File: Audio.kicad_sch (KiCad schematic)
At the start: 2 parts, among them J3 AudioJack3_Ground_SwitchTR, U3 WM8960CGEFL/RV

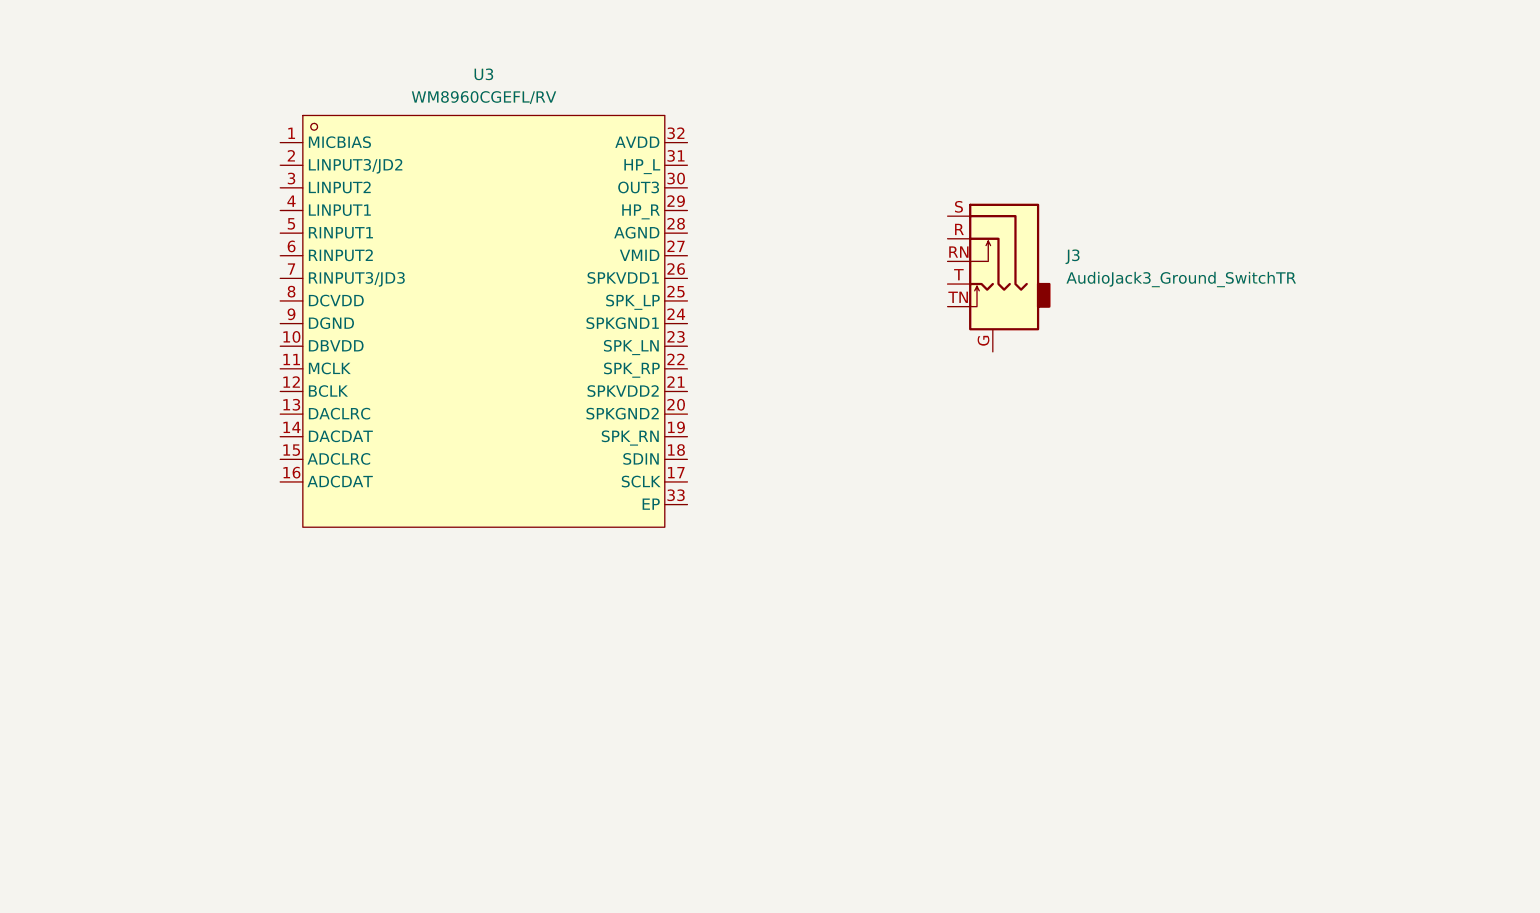
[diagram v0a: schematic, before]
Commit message: audio and display changes
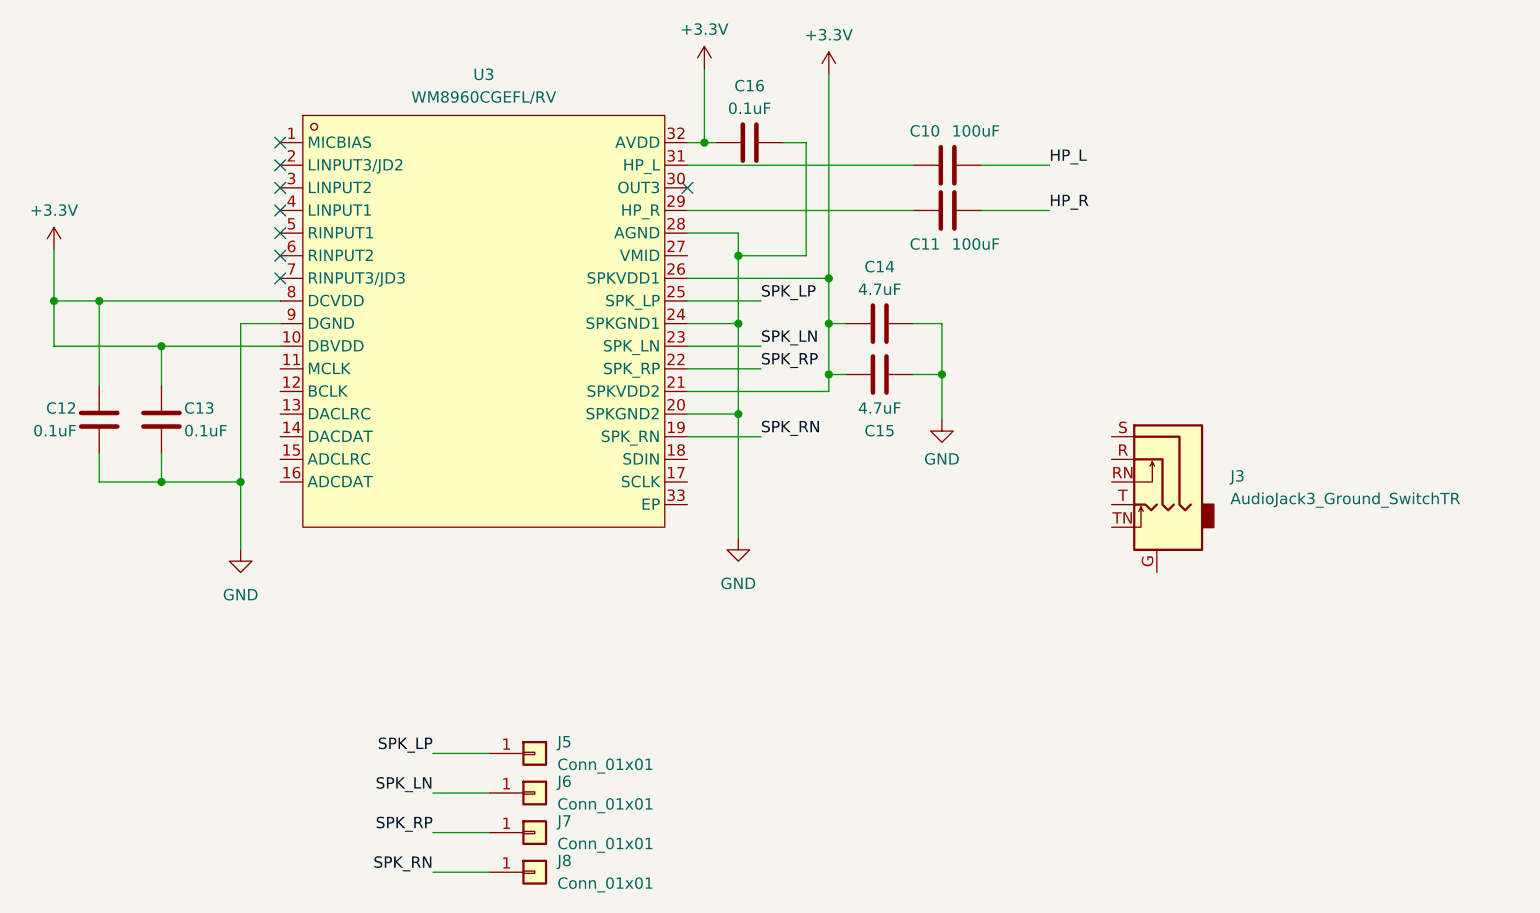
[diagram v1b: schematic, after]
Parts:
- added C10, C11: 100uF, symbol Device:C
- added C12, C13, C16: 0.1uF, symbol Device:C
- added C14, C15: 4.7uF, symbol Device:C
- added J5, J6, J7, J8: Conn_01x01, symbol Connector_Generic:Conn_01x01
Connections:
- net +3.3V: now reaches U3.10 (DBVDD)
- net +3.3V: now also U3.21 (SPKVDD2), U3.26 (SPKVDD1), U3.32 (AVDD), U3.8 (DCVDD), C12.1, C13.1, C14.1, C15.1, C16.1
- net SPK_RN: now reaches U3.19 (SPK_RN)
- net SPK_RN: now also J8.1 (Pin_1)
- net GND: now reaches U3.20 (SPKGND2)
- net GND: now also U3.24 (SPKGND1), U3.28 (AGND), U3.9 (DGND), C12.2, C13.2, C14.2, C15.2, C16.2
- net SPK_RP: now reaches U3.22 (SPK_RP)
- net SPK_RP: now also J7.1 (Pin_1)
- net SPK_LN: now reaches U3.23 (SPK_LN)
- net SPK_LN: now also J6.1 (Pin_1)
- net SPK_LP: now reaches U3.25 (SPK_LP)
- net SPK_LP: now also J5.1 (Pin_1)
- net at U3.29 (HP_R): now also C11.2
- net at U3.31 (HP_L): now also C10.1
- new net HP_L: C10.2
- new net HP_R: C11.1
- no-connect marks 0 -> 8
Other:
- moved on the sheet: J3

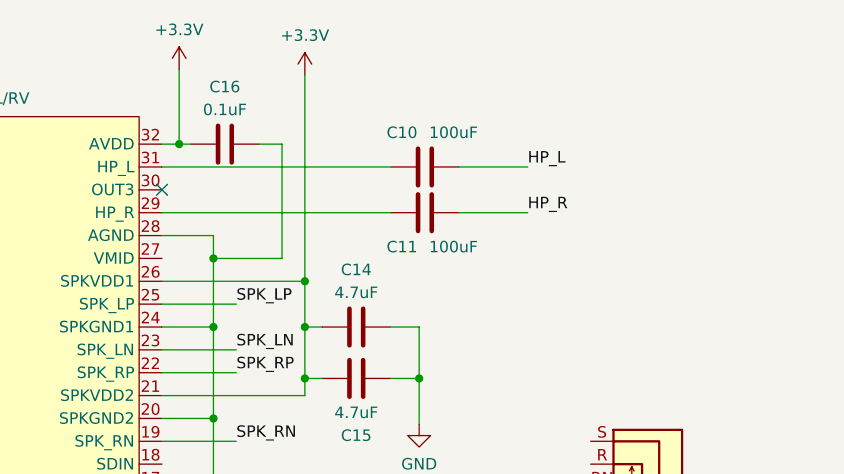
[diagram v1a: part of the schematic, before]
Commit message: more display things
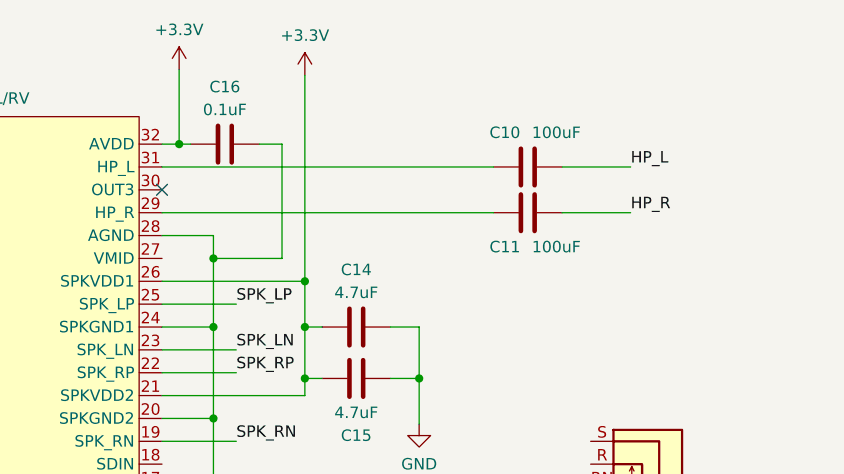
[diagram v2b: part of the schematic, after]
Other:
- moved on the sheet: C10, C11
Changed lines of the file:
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@@
     (stroke (width 0) (type default))
   )
-  (wire (pts (xy 145.415 59.69) (xy 153.035 59.69))
+  (wire (pts (xy 156.845 59.69) (xy 164.465 59.69))
     (stroke (width 0) (type default))
   )
@@
     (stroke (width 0) (type default))
   )
-  (wire (pts (xy 145.415 64.77) (xy 153.035 64.77))
+  (wire (pts (xy 156.845 64.77) (xy 164.465 64.77))
     (stroke (width 0) (type default))
   )
@@
     (stroke (width 0) (type default))
   )
-  (wire (pts (xy 112.395 64.77) (xy 137.795 64.77))
+  (wire (pts (xy 112.395 64.77) (xy 149.225 64.77))
     (stroke (width 0) (type default))
   )
@@
     (stroke (width 0) (type default))
   )
-  (wire (pts (xy 112.395 59.69) (xy 137.795 59.69))
+  (wire (pts (xy 112.395 59.69) (xy 149.225 59.69))
     (stroke (width 0) (type default))
   )
@@
     (effects (font (size 1.27 1.27)) (justify left bottom))
   )
-  (label "HP_R" (at 153.035 64.77 0) (fields_autoplaced)
+  (label "HP_R" (at 164.465 64.77 0) (fields_autoplaced)
     (effects (font (size 1.27 1.27)) (justify left bottom))
   )
-  (label "HP_L" (at 153.035 59.69 0) (fields_autoplaced)
+  (label "HP_L" (at 164.465 59.69 0) (fields_autoplaced)
     (effects (font (size 1.27 1.27)) (justify left bottom))
   )
@@
     )
   )
-  (symbol (lib_id "Device:C") (at 141.605 59.69 90) (unit 1)
+  (symbol (lib_id "Device:C") (at 153.035 59.69 90) (unit 1)
     (in_bom yes) (on_board yes) (dnp no)
-    (property "Reference" "C10" (at 139.065 55.88 90)
-      (effects (font (size 1.27 1.27)))
-    )
-    (property "Value" "100uF" (at 144.78 55.88 90)
-      (effects (font (size 1.27 1.27)))
-    )
-    (property "Footprint" "" (at 145.415 58.7248 0)
-      (effects (font (size 1.27 1.27)) hide)
-    )
-    (property "Datasheet" "~" (at 141.605 59.69 0)
+    (property "Reference" "C10" (at 150.495 55.88 90)
+      (effects (font (size 1.27 1.27)))
+    )
+    (property "Value" "100uF" (at 156.21 55.88 90)
+      (effects (font (size 1.27 1.27)))
+    )
+    (property "Footprint" "" (at 156.845 58.7248 0)
+      (effects (font (size 1.27 1.27)) hide)
+    )
+    (property "Datasheet" "~" (at 153.035 59.69 0)
       (effects (font (size 1.27 1.27)) hide)
     )
@@
     )
   )
-  (symbol (lib_id "Device:C") (at 141.605 64.77 270) (unit 1)
+  (symbol (lib_id "Device:C") (at 153.035 64.77 270) (unit 1)
     (in_bom yes) (on_board yes) (dnp no)
-    (property "Reference" "C11" (at 139.065 68.58 90)
-      (effects (font (size 1.27 1.27)))
-    )
-    (property "Value" "100uF" (at 144.78 68.58 90)
-      (effects (font (size 1.27 1.27)))
-    )
-    (property "Footprint" "" (at 137.795 65.7352 0)
-      (effects (font (size 1.27 1.27)) hide)
-    )
-    (property "Datasheet" "~" (at 141.605 64.77 0)
-      (effects (font (size 1.27 1.27)) hide)
-    )
+    (property "Reference" "C11" (at 150.495 68.58 90)
+      (effects (font (size 1.27 1.27)))
+    )
+    (property "Value" "100uF" (at 156.21 68.58 90)
+      (effects (font (size 1.27 1.27)))
+    )
+    (property "Footprint" "" (at 149.225 65.7352 0)
+      (effects (font (size 1.27 1.27)) hide)
+    )
+    (property "Datasheet" "~" (at 153.035 64.77 0)
+      (effects (font (size 1.27 1.27)) hide)
+    )
